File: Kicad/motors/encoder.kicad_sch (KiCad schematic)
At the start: 28 parts, among them IC301 SN74LVC2G17, IC302 SN74LVC2G17, IC303 TTE-OPB610, IC304 TTE-OPB610, IC305 TTE-OPB610, IC306 TTE-OPB610, IC307 LM3480-33, K301 Front, K302 Rear, Q301 NEXPERIA-BC846BS, Q302 NEXPERIA-BC846BS

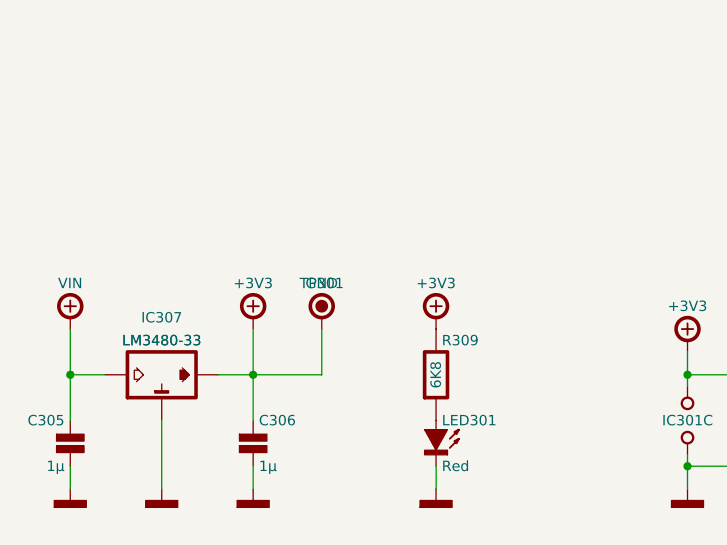
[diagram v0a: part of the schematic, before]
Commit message: Update
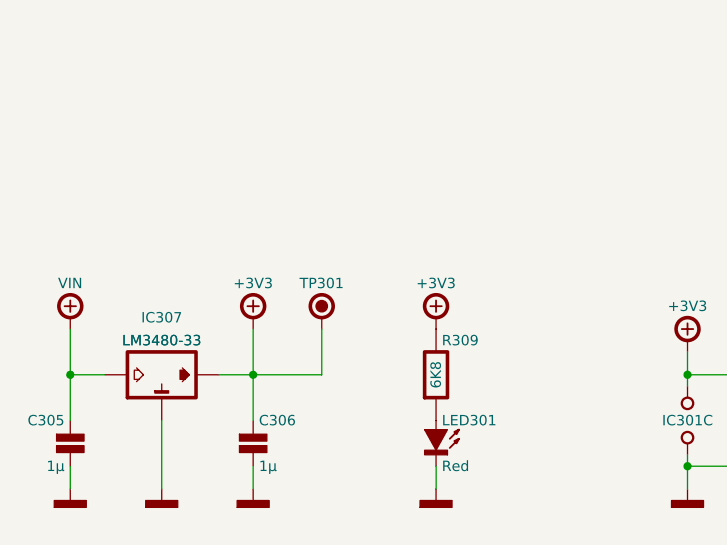
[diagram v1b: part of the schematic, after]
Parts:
- TP301: footprint tronixio:HARWIN-S1751 -> tronixio:zzzHARWIN-S1751; Name GND -> (none)
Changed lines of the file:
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@@
       (effects (font (size 1 1)) hide)
     )
-    (property "Footprint" "tronixio:HARWIN-S1751" (id 2) (at 53.34 177.8 0)
+    (property "Footprint" "tronixio:zzzHARWIN-S1751" (id 2) (at 53.34 177.8 0)
       (effects (font (size 1 1)) hide)
     )
@@
       (effects (font (size 1 1)) hide)
     )
-    (property "Name" "GND" (id 5) (at 53.34 162.56 0)
-      (effects (font (size 1.15 1.15)))
-    )
     (pin "1")
